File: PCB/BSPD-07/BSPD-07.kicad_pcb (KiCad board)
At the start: 2 copper layers, 78.7 x 30 mm, 17 parts, among them IC1 LM393LVQDRQ1, IC2 LM393LVQDRQ1, IC3 LM393LVQDRQ1, J1 DTM13-12PA

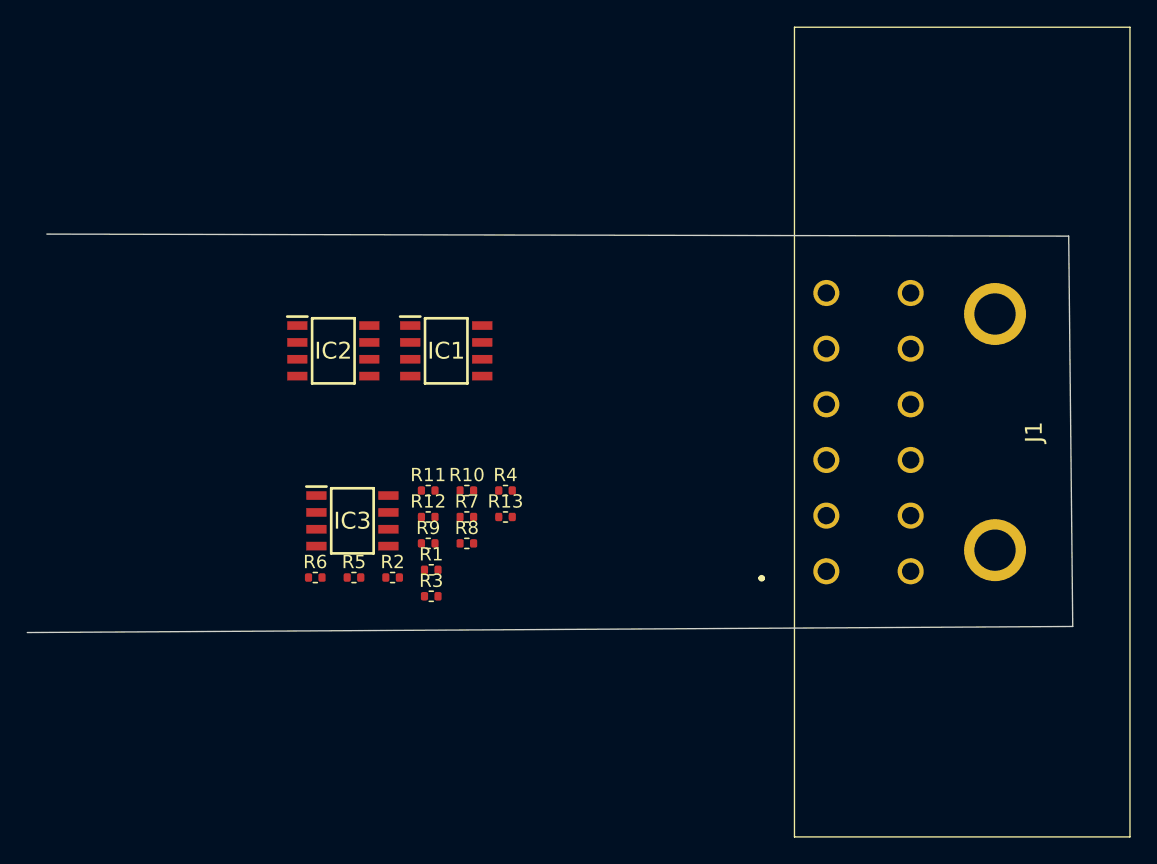
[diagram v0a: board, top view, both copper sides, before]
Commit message: New revision with LDO40L
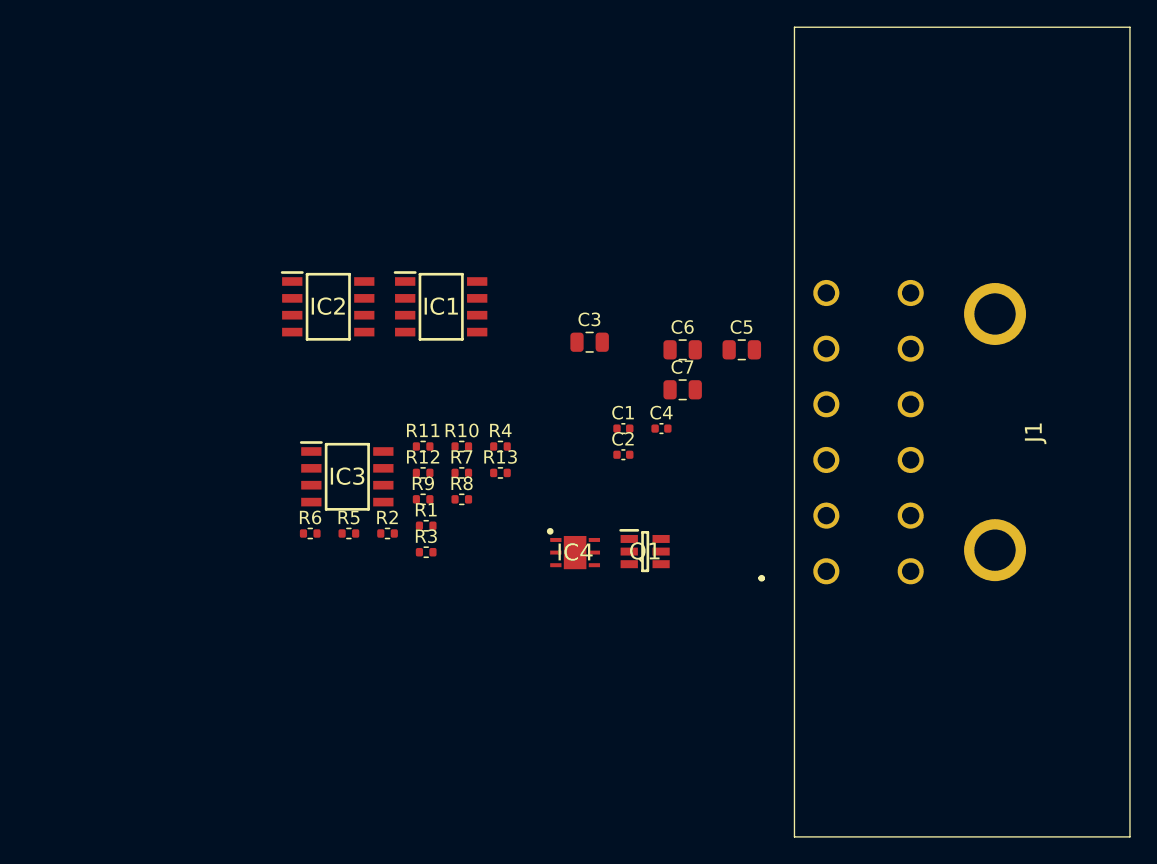
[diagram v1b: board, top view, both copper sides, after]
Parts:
- added C1: 0.1uF, Capacitor_SMD:C_0402_1005Metric, F.Cu at (66.7, 72.6)
- added C2: 0.1uF, Capacitor_SMD:C_0402_1005Metric, F.Cu at (66.7, 74.5)
- added C3: 10u, Capacitor_SMD:C_0805_2012Metric, F.Cu at (64.2, 66.1)
- added C4: 0.1uF, Capacitor_SMD:C_0402_1005Metric, F.Cu at (69.6, 72.6)
- added C5: 10uF, Capacitor_SMD:C_0805_2012Metric, F.Cu at (75.6, 66.6)
- added C6: 1uF, Capacitor_SMD:C_0805_2012Metric, F.Cu at (71.2, 66.6)
- added C7: 4.7uF, Capacitor_SMD:C_0805_2012Metric, F.Cu at (71.2, 69.6)
- added IC4: LDO40LPU50RY, BSPD_07:SON95P300X300X90-7N-D, F.Cu at (63.1, 81.9)
- added Q1: RSQ025P03HZGTR, BSPD_07:SOT95P280X100-6N, F.Cu at (68.3, 81.8)
- moved R8 3.34 mm to (54.5, 77.9)
- moved R9 3.34 mm to (51.6, 77.9)
- moved IC1 3.34 mm to (53.0, 63.4)
- moved IC2 3.34 mm to (44.5, 63.4)
- moved IC3 3.34 mm to (45.9, 76.2)
- moved R1 3.34 mm to (51.9, 79.9)
- moved R10 3.34 mm to (54.5, 73.9)
- moved R11 3.34 mm to (51.6, 73.9)
- moved R12 3.34 mm to (51.6, 75.9)
- moved R13 3.34 mm to (57.4, 75.9)
- moved R2 3.34 mm to (48.9, 80.5)
- moved R3 3.34 mm to (51.9, 81.9)
- moved R4 3.34 mm to (57.4, 73.9)
- moved R5 3.34 mm to (46.0, 80.5)
- moved R6 3.34 mm to (43.1, 80.5)
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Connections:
- net ERROR_CUR renamed ERR_CURRENT
- IC1 pad 3: Net-(IC1-Pad3) -> TPS_TRIG
- IC2 pad 3: Net-(IC2-Pad3) -> BRAKE_TRIG
- IC3 pad 1: unconnected-(IC3-Pad1) -> Net-(IC3-Pad1)
- IC3 pad 6: unconnected-(IC3-Pad6) -> Net-(IC3-Pad6)
- J1 pad 7: unconnected-(J1-Pad7) -> BRAKE_TRIG
- J1 pad 8: unconnected-(J1-Pad8) -> TPS_TRIG
- R3 pad 2: Net-(IC1-Pad3) -> TPS_TRIG
- R5 pad 2: Net-(IC2-Pad3) -> BRAKE_TRIG
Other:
- board outline removed
